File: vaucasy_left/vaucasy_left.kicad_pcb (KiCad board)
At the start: 2 copper layers, 153.2 x 136.5 mm, 105 parts, among them J1 USB_C, J2 OLED_128x32, J4 Trackball, J5 HC-05 BT, J6 DEBUG, SW1 SW_SPDT, SW2 SW_Push, SW3 RotaryEncoder_Switch, U1 STM32F401RET6, U2 USBLC6-2SC6, U3 XC6206, U4 TRRS, Y1 8MHz

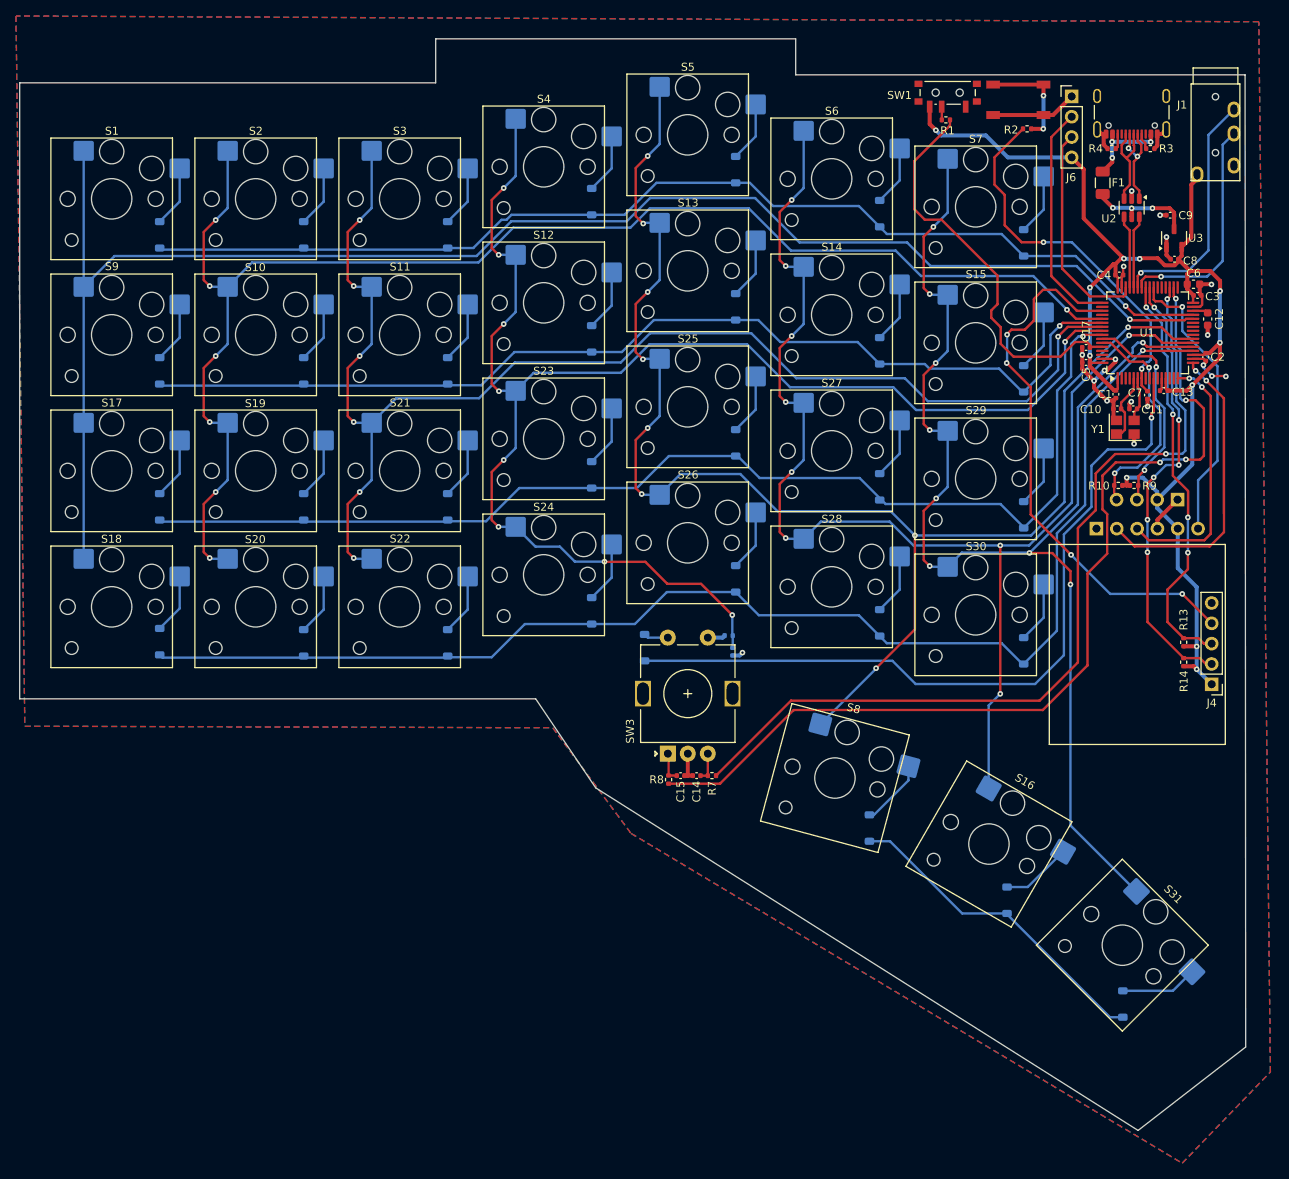
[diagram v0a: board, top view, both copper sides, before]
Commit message: ordered
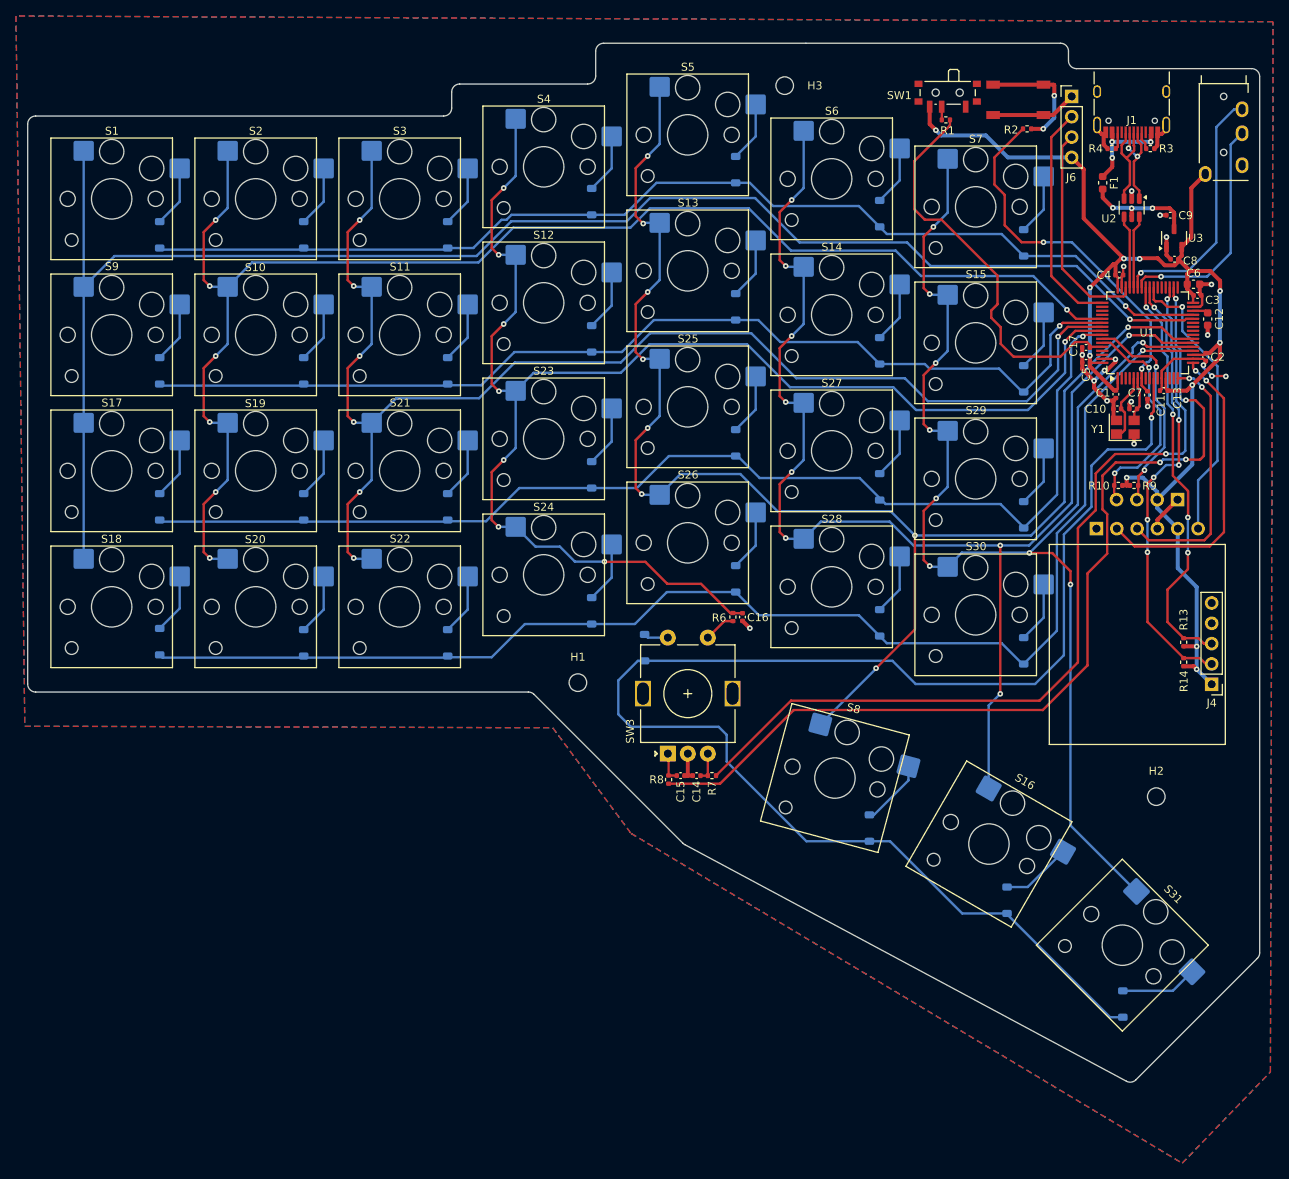
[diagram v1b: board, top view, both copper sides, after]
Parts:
- added H1: MountingHole, MountingHole:MountingHole_2.2mm_M2, F.Cu at (93.8, 107.8)
- added H2: MountingHole, MountingHole:MountingHole_2.2mm_M2, F.Cu at (166.1, 122.1)
- added H3: MountingHole, MountingHole:MountingHole_2.2mm_M2, F.Cu at (119.6, 33.2)
- C16, R6: moved to F.Cu
- F1: footprint Fuse:Fuse_1206_3216Metric -> Fuse:Fuse_0603_1608Metric
- J1: footprint Connector_USB:USB_C_Receptacle_GCT_USB4105-xx-A_16P_TopMnt_Horizontal -> Connector_USB:USB_C_Receptacle_HRO_TYPE-C-31-M-12
- J5: footprint Connector_PinSocket_2.54mm:PinSocket_1x06_P2.54mm_Horizontal -> Connector_PinSocket_2.54mm:PinSocket_1x06_P2.54mm_Vertical
- moved C16 4.50 mm to (114.3, 99.6)
- moved R6 2.38 mm to (113.2, 99.6), turned to -90 degrees
- moved U4 1.03 mm to (174.5, 33.0)
- moved J1 0.59 mm to (163.0, 35.0)
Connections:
- D16 pad 1: LROW4 -> LRow 4
- D31 pad 1: LROW4 -> LRow 4
- D8 pad 1: LROW4 -> LRow 4
- J4 pad 4: LTRACK_INT -> unconnected-(J4-INT-Pad4)
- U1 pad 51: LTRACK_INT -> unconnected-(U1-PC10-Pad51)
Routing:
- net LRow 4: track 97.2 -> 186.5 mm
- net LTRACK_INT: track 68.9 -> 0.00 mm, vias 4 -> 0
- net LROW4: track 40.8 -> 0.00 mm
- net GND: track 69.8 -> 75.2 mm
- net LColumn 3: track 183.6 -> 180.6 mm, vias 9 -> 8
- net Net-(R2-Pad2): track 13.4 -> 15.2 mm
- net Net-(R6-Pad2): track 2.20 -> 3.99 mm
- net LUART1_RX: track 30.5 -> 31.6 mm
- net VBUS: track 11.1 -> 11.7 mm
- net +5V: track 13.2 -> 13.9 mm
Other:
- board size 153.2 x 136.5 mm -> 154 x 129.9 mm
